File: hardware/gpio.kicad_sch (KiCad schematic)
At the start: 23 parts, among them J3 HDMI_C_1.3, U1 ECP5U_12_CABGA256, U5 PCA9306DC1

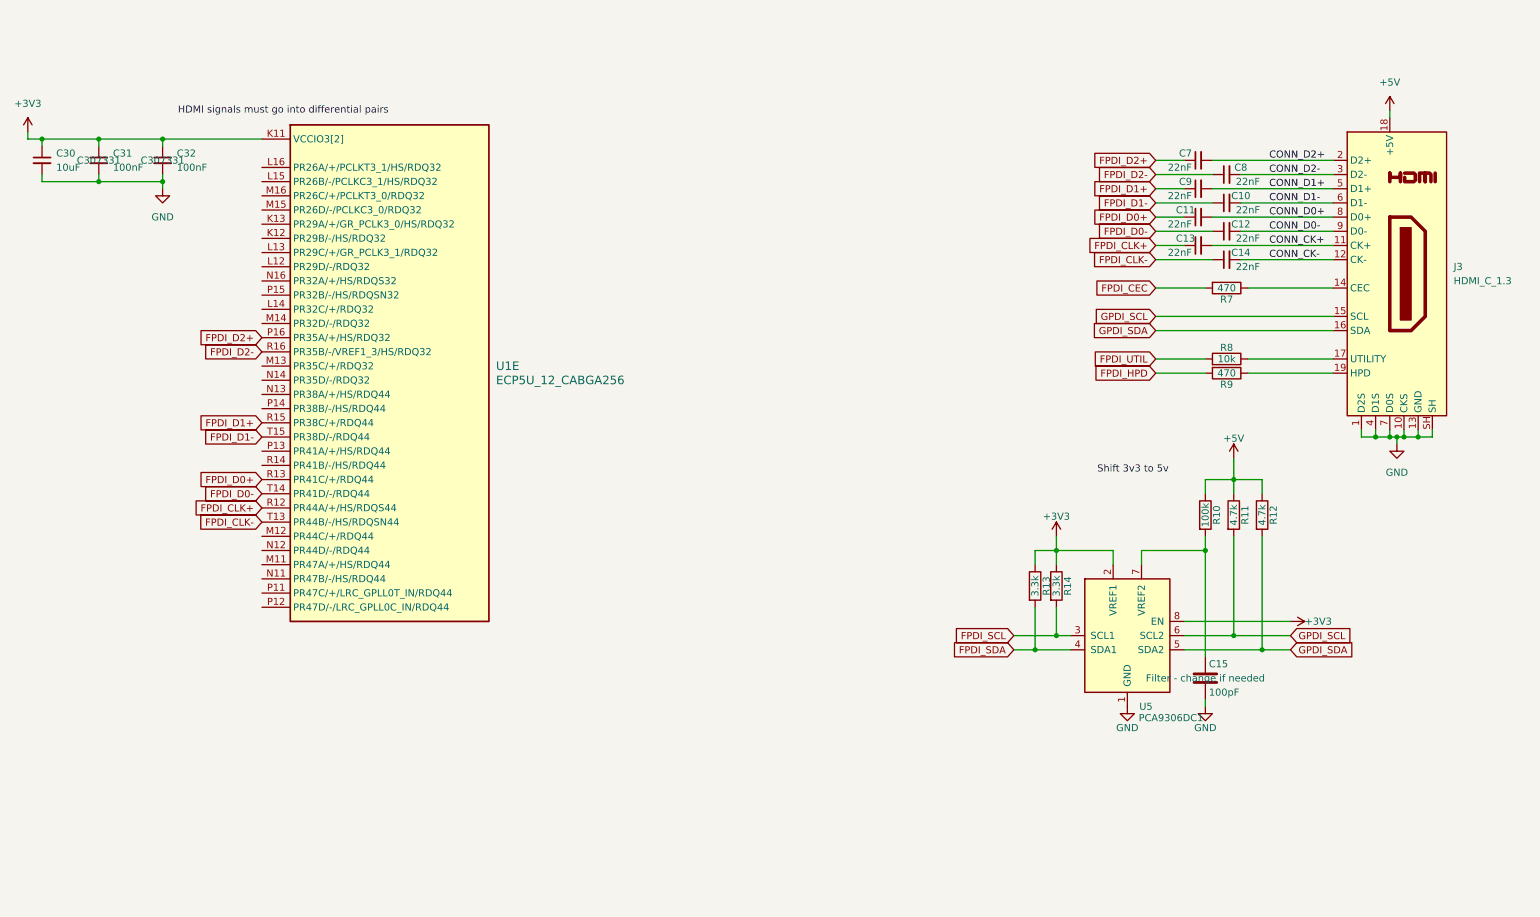
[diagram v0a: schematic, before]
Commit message: V1.0 Final Revision and Readme documentation
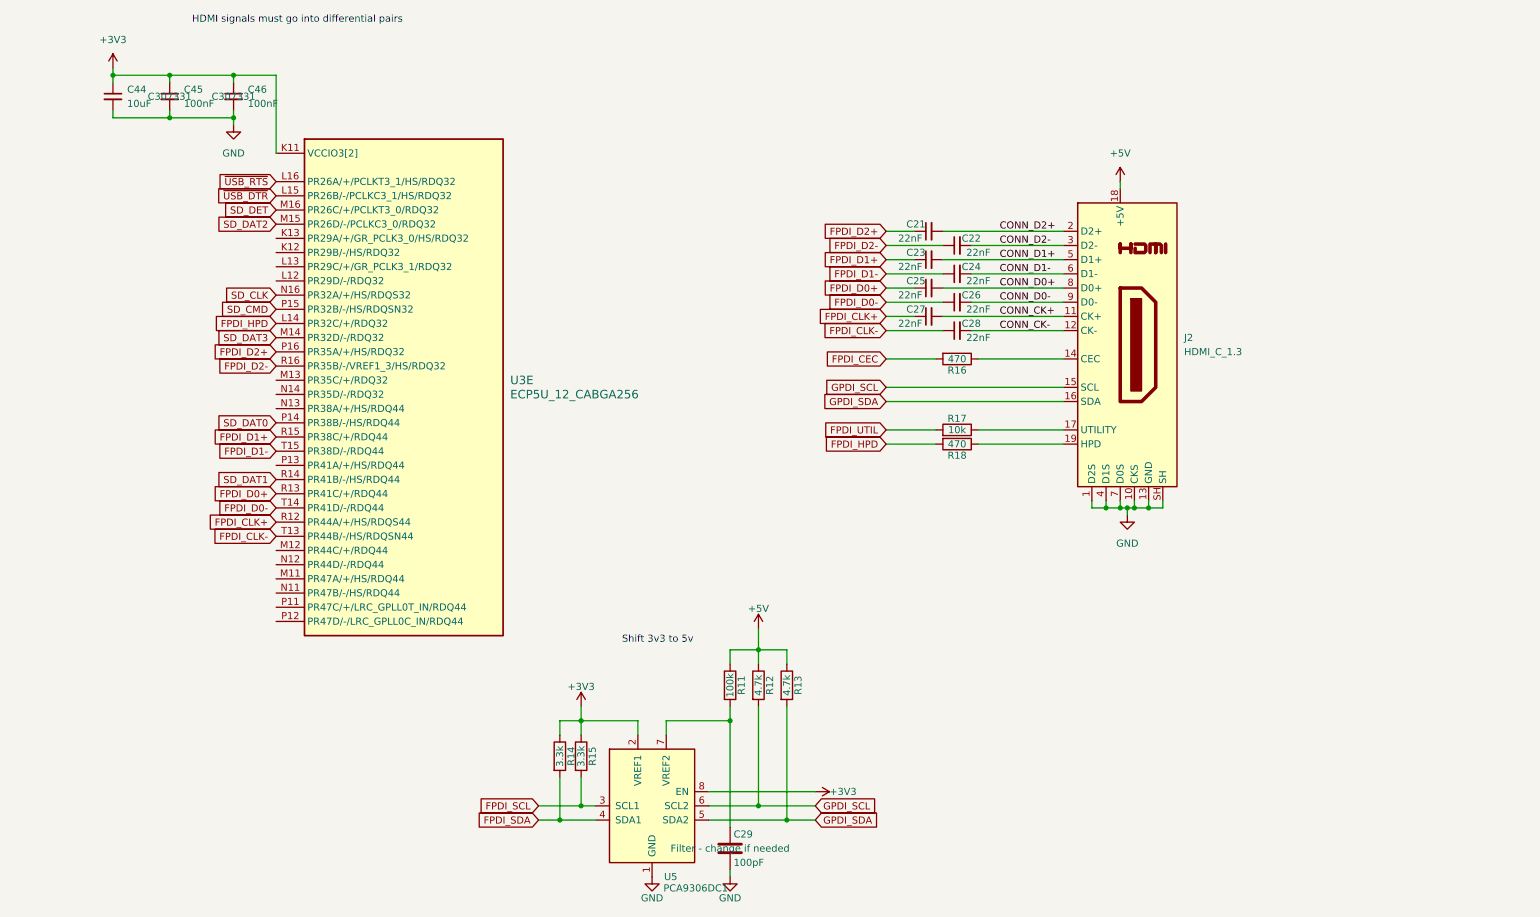
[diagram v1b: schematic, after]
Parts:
- removed U1: ECP5U_12_CABGA256, Package_BGA:BGA-256_14.0x14.0mm_Layout16x16_P0.8mm_Ball0.45mm_Pad0.32mm_NSMD, symbol josh:ECP5U_12_CABGA256
- added U3: ECP5U_12_CABGA256, Package_BGA:BGA-256_14.0x14.0mm_Layout16x16_P0.8mm_Ball0.45mm_Pad0.32mm_NSMD, symbol josh:ECP5U_12_CABGA256
- renumbered C7 to C21, C8 to C22, C9 to C23, C10 to C24, C11 to C25, C12 to C26, C13 to C27, C14 to C28, C15 to C29, C30 to C44, C31 to C45, C32 to C46, J3 to J2, R10 to R11, R11 to R12, R12 to R13, R13 to R14, R14 to R15, R7 to R16, R8 to R17, R9 to R18
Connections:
- net +3V3: now also U3.K11 (VCCIO3[2]), U3.L11 (VCCIO3[2])
- net FPDI_CLK+: now also U3.R12 (PR44A/+/HS/RDQS44)
- net FPDI_CLK-: now also U3.T13 (PR44B/-/HS/RDQSN44)
- net FPDI_D0+: now also U3.R13 (PR41C/+/RDQ44)
- net FPDI_D0-: now also U3.T14 (PR41D/-/RDQ44)
- net FPDI_D1+: now also U3.R15 (PR38C/+/RDQ44)
- net FPDI_D1-: now also U3.T15 (PR38D/-/RDQ44)
- net FPDI_D2+: now also U3.P16 (PR35A/+/HS/RDQ32)
- net FPDI_D2-: now also U3.R16 (PR35B/-/VREF1_3/HS/RDQ32)
- net FPDI_HPD: now also U3.L14 (PR32C/+/RDQ32)
- new net SD_CLK: U3.N16 (PR32A/+/HS/RDQS32)
- new net SD_CMD: U3.P15 (PR32B/-/HS/RDQSN32)
- new net SD_DAT0: U3.P14 (PR38B/-/HS/RDQ44)
- new net SD_DAT1: U3.R14 (PR41B/-/HS/RDQ44)
- new net SD_DAT2: U3.M15 (PR26D/-/PCLKC3_0/RDQ32)
- new net SD_DAT3: U3.M14 (PR32D/-/RDQ32)
- new net SD_DET: U3.M16 (PR26C/+/PCLKT3_0/RDQ32)
- new net ~{USB_DTR}: U3.L15 (PR26B/-/PCLKC3_1/HS/RDQ32)
- new net ~{USB_RTS}: U3.L16 (PR26A/+/PCLKT3_1/HS/RDQ32)
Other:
- moved on the sheet: C21, C22, C23, C24, C25, C26, C27, C28, C29, C44, C45, C46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
